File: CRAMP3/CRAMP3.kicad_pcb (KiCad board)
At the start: 2 copper layers, 20 parts, among them M101 POLOLU_SOCKET, M102 POLOLU_SOCKET, P101 HEADER_3X2, P102 HEADER_3X2, P103 HEADER_3X2, P104 X-MOT, P105 Y-MOT, P106 Z-MOT, P107 HEADER_4X2, P108 Aux-3, P109 HEADER_3X2, U101 SM_DRIVER, U102 SM_DRIVER, U103 SM_DRIVER

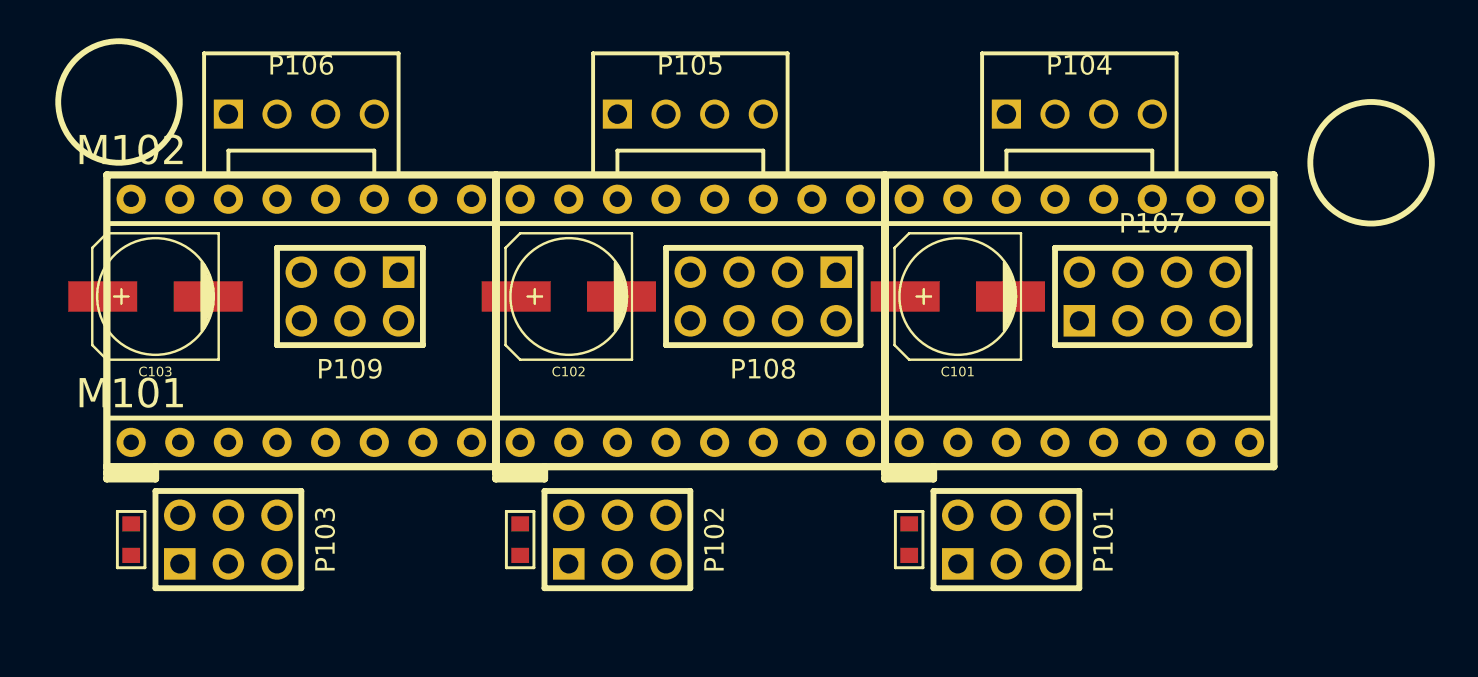
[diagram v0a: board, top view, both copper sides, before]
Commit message: CRAMP3 updates, PCB mostly complete
Signed-off-by: Charles Steinkuehler <charles@steinkuehler.net>
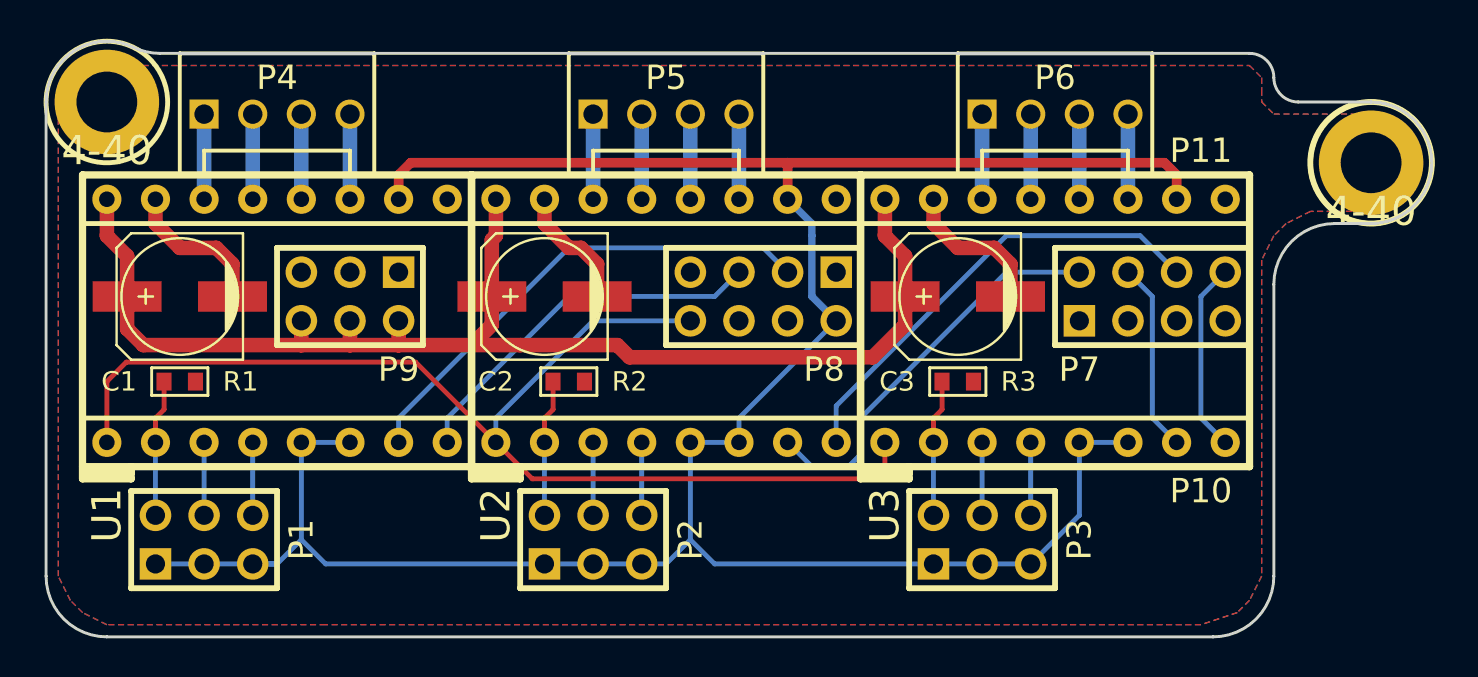
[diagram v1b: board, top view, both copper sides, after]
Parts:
- removed P103: HEADER_3X2, pin_strip_3x2
- added M1: 4-40, MTH_4-40, F.Cu at (77.5, 59.7)
- added M2: 4-40, MTH_4-40, F.Cu at (143.5, 62.9)
- added P3: HEADER_3X2, pin_strip_3x2, F.Cu at (123.2, 82.5)
- moved R3 44.0 mm to (121.9, 74.3), turned to 0 degrees
- moved P4 41.9 mm to (86.4, 60.3)
- moved U1 41.9 mm to (86.4, 77.5)
- moved C3 41.9 mm to (121.9, 69.8)
- moved P1 41.9 mm to (82.5, 82.5)
- moved C1 40.6 mm to (81.3, 69.8)
- moved P6 39.4 mm to (127.0, 60.3)
- moved U3 39.4 mm to (127.0, 77.5)
- moved R1 39.0 mm to (81.3, 74.3), turned to 0 degrees
- moved R2 8.64 mm to (101.6, 74.3), turned to 0 degrees
- moved C2 1.27 mm to (100.3, 69.8)
- moved P10 1.27 mm to (77.5, 77.5)
- moved P11 1.27 mm to (77.5, 64.8)
- moved P2 1.27 mm to (102.9, 82.5)
- moved P5 1.27 mm to (106.7, 60.3)
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- renumbered C101 to C1, C102 to C2, C103 to C3, P101 to P1, M101 to P10, M102 to P11, P102 to P2, P104 to P4, P105 to P5, P106 to P6, P107 to P7, P108 to P8, P109 to P9, R101 to R1, R102 to R2, R103 to R3, U101 to U1, U102 to U2, U103 to U3
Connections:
- P7 pad 2: (no net) -> STEP_1
- P7 pad 4: (no net) -> STEP_2
- P7 pad 6: (no net) -> DIR_1
- P7 pad 8: (no net) -> DIR_2
- P8 pad 3: (no net) -> STEP_0
- P8 pad 5: (no net) -> DIR_0
- U1 pad 7: (no net) -> STEP_0
- U1 pad 8: (no net) -> DIR_0
- U2 pad 7: (no net) -> STEP_1
- U2 pad 8: (no net) -> DIR_1
- U3 pad 7: (no net) -> STEP_2
- U3 pad 8: (no net) -> DIR_2
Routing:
- net +3.3V: track 0.00 -> 135.7 mm
- net +V_MOTOR: track 0.00 -> 68.1 mm
- net ENAn: track 0.00 -> 61.8 mm
- net STEP_0: track 0.00 -> 25.8 mm
- net DIR_1: track 0.00 -> 24.2 mm
- net GND: track 0.00 -> 22.3 mm
- net STEP_1: track 0.00 -> 21.1 mm
- net DIR_0: track 0.00 -> 19.7 mm
- net STEP_2: track 0.00 -> 9.94 mm
- net DIR_2: track 0.00 -> 9.94 mm
- net N-0000040: track 0.00 -> 7.17 mm
- net N-0000043: track 0.00 -> 7.17 mm
- net N-0000042: track 0.00 -> 7.17 mm
- net N-000009: track 0.00 -> 4.44 mm
- net N-0000041: track 0.00 -> 4.44 mm
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- added copper zone on B.Cu, net GND
- added copper zone on F.Cu, net GND
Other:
- board outline added: 72.4 x 31.1 mm
